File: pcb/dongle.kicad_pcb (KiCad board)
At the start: 2 copper layers, 12 x 16 mm, 28 parts, among them J1 USB_A, J2 Conn_01x01_Pin, J3 Conn_01x01_Pin, J4 Conn_01x01_Pin, J5 Conn_01x01_Pin, U3 nRF52833_QDxx, Y1 Crystal_GND24, Y2 Crystal_Small

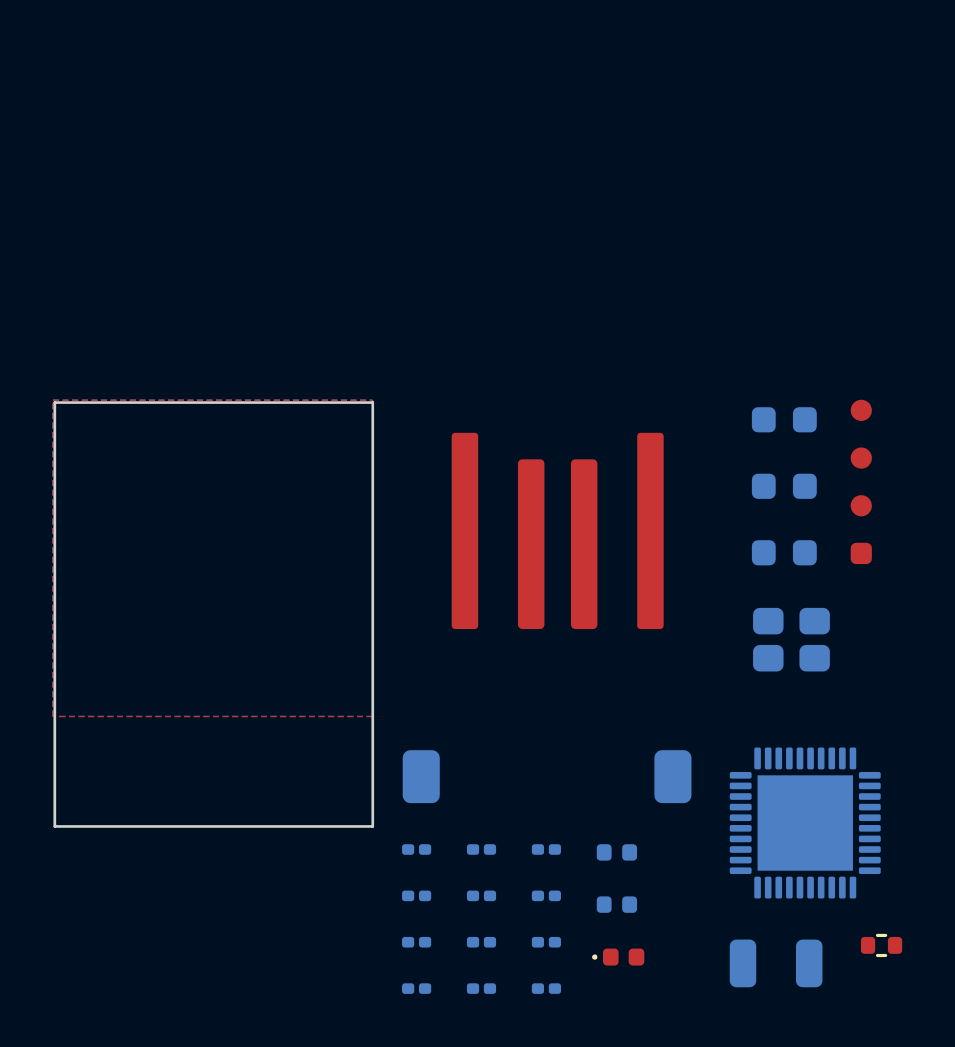
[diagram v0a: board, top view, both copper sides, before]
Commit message: update pcb
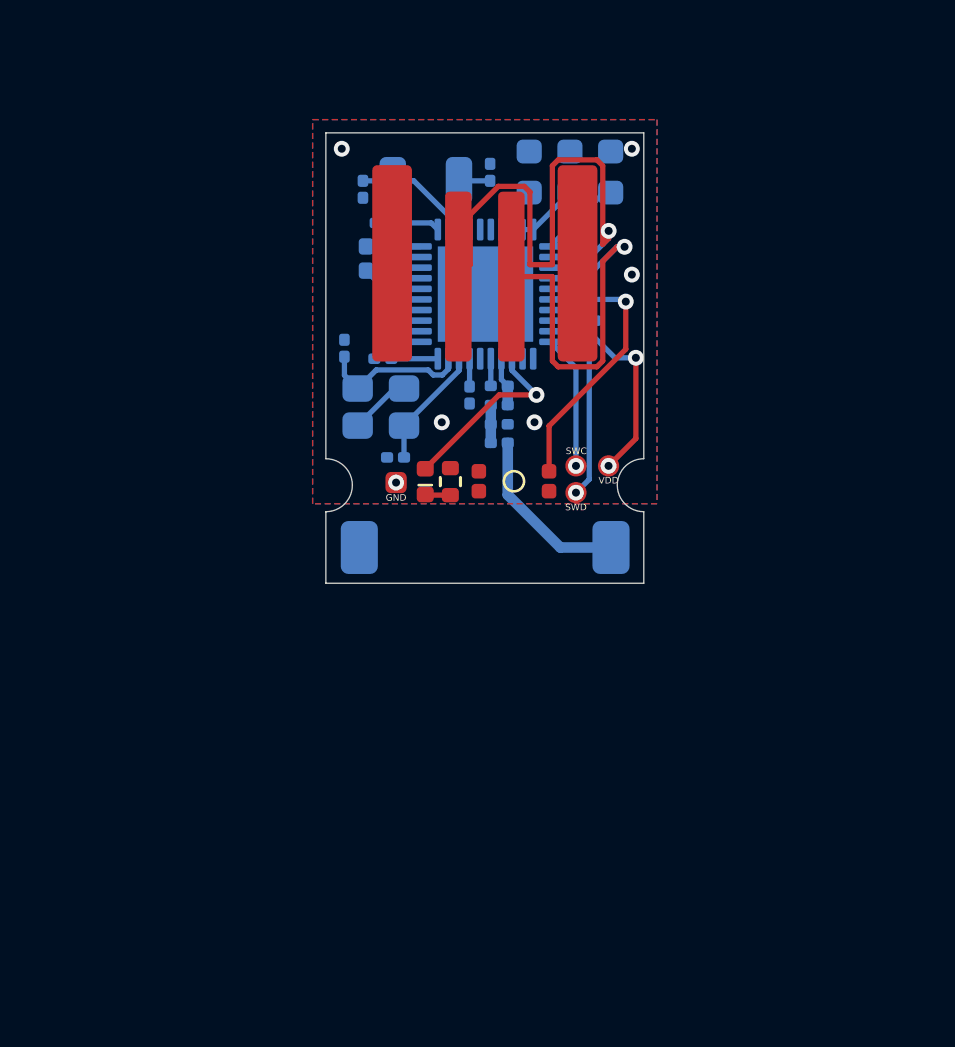
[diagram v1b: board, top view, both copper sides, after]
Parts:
- added SW1: SW_Push_45deg, dongle:SKTAAAE010, F.Cu at (157.1, 96.2)
- moved Y2 32.4 mm to (153.8, 84.8), turned to 180 degrees
- moved C16 27.6 mm to (151.4, 85.1), turned to -90 degrees
- moved C15 25.6 mm to (156.2, 84.5), turned to -90 degrees
- moved C13 25.6 mm to (152.0, 88.2), turned to 180 degrees
- moved C12 24.6 mm to (152.0, 87.3), turned to 180 degrees
- moved C11 24.1 mm to (152.2, 91.5), turned to 180 degrees
- moved C5 23.9 mm to (152.2, 86.4), turned to 180 degrees
- moved R1 23.9 mm to (154.7, 96.2), turned to 90 degrees
- moved U3 23.3 mm to (156.0, 89.1), turned to 90 degrees
- moved C7 22.1 mm to (159.8, 90.1)
- moved C4 21.5 mm to (156.5, 94.0), turned to 180 degrees
- moved C3 21.2 mm to (156.5, 92.5), turned to 180 degrees
- moved C2 20.8 mm to (150.7, 91.1), turned to 90 degrees
- moved L2 20.7 mm to (156.5, 94.7), turned to 180 degrees
- moved C10 20.7 mm to (155.4, 92.9), turned to -90 degrees
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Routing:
- net D-: track 0.00 -> 21.1 mm, vias 0 -> 1
- net D+: track 0.00 -> 14.8 mm, vias 0 -> 1
- net VDD: track 0.00 -> 12.9 mm, vias 0 -> 2
- net RESET: track 0.00 -> 10.5 mm, vias 0 -> 1
- net SWD: track 0.00 -> 7.15 mm, vias 0 -> 1
- net LED: track 0.00 -> 7.10 mm, vias 0 -> 1
- net Net-(AE1-A): track 0.00 -> 6.68 mm
- net XC2: track 0.00 -> 5.68 mm
- net SWC: track 0.00 -> 5.09 mm, vias 0 -> 1
- net GND: track 0.00 -> 4.70 mm, vias 0 -> 6
- net XC1: track 0.00 -> 4.58 mm
- net XL1: track 0.00 -> 4.30 mm
- net DECUSB: track 0.00 -> 3.13 mm
- net XL2: track 0.00 -> 3.01 mm
- net VBUS: track 0.00 -> 2.37 mm
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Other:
- board size 12 x 16 mm -> 12 x 17 mm

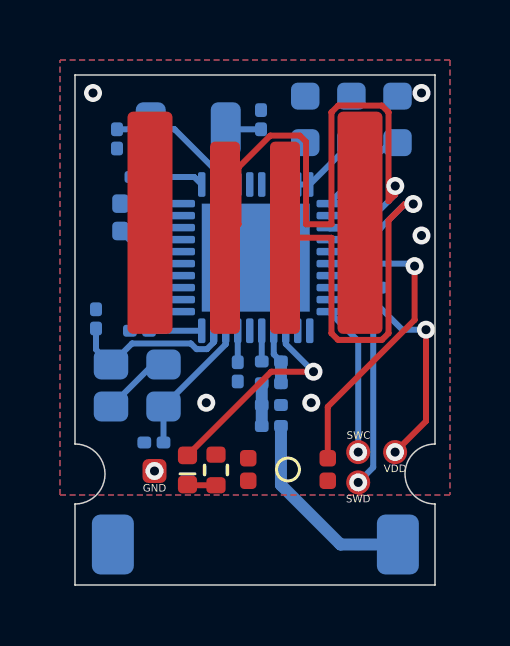
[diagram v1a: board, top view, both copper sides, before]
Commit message: some fix
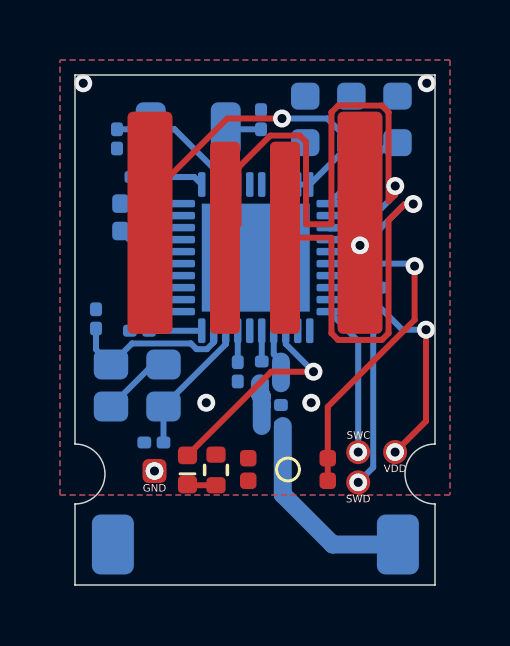
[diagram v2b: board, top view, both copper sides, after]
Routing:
- net VBUS: track 2.37 -> 11.4 mm, vias 0 -> 1
- net RESET: track 10.5 -> 11.2 mm
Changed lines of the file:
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@@
 			(outputformat 1)
 			(mirror no)
-			(drillshape 1)
+			(drillshape 0)
 			(scaleselection 1)
-			(outputdirectory "")
+			(outputdirectory "../../../../../dongle_gerber/")
 		)
 	)
@@
 	)
 	(footprint "dongle:QFN-40-1EP_5x5mm_P0.4mm_EP3.6x3.6mm"
-		(locked yes)
 		(layer "F.Cu")
 		(at 156.025 89.0875 90)
@@
 	)
 	(via micro
-		(at 150.6 83.6)
+		(at 159.5 88.68)
 		(size 0.6)
 		(drill 0.3)
 		(layers "F.Cu" "B.Cu")
-		(free yes)
 		(net 1)
 	)
 	(via micro
-		(at 157.875 93.925)
+		(at 150.275 83.275)
 		(size 0.6)
 		(drill 0.3)
@@
 	)
 	(via micro
-		(at 161.55 88.35)
+		(at 157.875 93.925)
 		(size 0.6)
 		(drill 0.3)
@@
 	)
 	(via micro
-		(at 161.55 83.6)
+		(at 161.724999 83.275)
 		(size 0.6)
 		(drill 0.3)
@@
 	)
 	(segment
+		(start 156.9 84.45)
+		(end 155.078756 84.45)
+		(width 0.2)
+		(layer "F.Cu")
+		(net 2)
+	)
+	(segment
+		(start 152.5 87.028756)
+		(end 152.5 87.925)
+		(width 0.2)
+		(layer "F.Cu")
+		(net 2)
+	)
+	(segment
+		(start 155.078756 84.45)
+		(end 152.5 87.028756)
+		(width 0.2)
+		(layer "F.Cu")
+		(net 2)
+	)
+	(via micro
+		(at 156.9 84.45)
+		(size 0.6)
+		(drill 0.3)
+		(layers "F.Cu" "B.Cu")
+		(net 2)
+	)
+	(segment
+		(start 159.2125 85.255)
+		(end 158.4075 84.45)
+		(width 0.2)
+		(layer "B.Cu")
+		(net 2)
+	)
+	(segment
+		(start 158.4075 84.45)
+		(end 156.9 84.45)
+		(width 0.2)
+		(layer "B.Cu")
+		(net 2)
+	)
+	(segment
 		(start 159.2125 85.255)
 		(end 159.2125 85.2625)
@@
 	)
 	(segment
-		(start 156.865 94.7)
-		(end 156.865 96.665)
-		(width 0.4)
+		(start 160.7625 98.65)
+		(end 158.59 98.65)
+		(width 0.6)
 		(layer "B.Cu")
 		(net 6)
 	)
 	(segment
-		(start 158.85 98.65)
-		(end 160.7625 98.65)
-		(width 0.4)
+		(start 158.59 98.65)
+		(end 156.926 96.986)
+		(width 0.6)
 		(layer "B.Cu")
 		(net 6)
 	)
 	(segment
-		(start 156.865 96.665)
-		(end 158.85 98.65)
-		(width 0.4)
+		(start 156.926 96.986)
+		(end 156.926 94.7)
+		(width 0.6)
 		(layer "B.Cu")
 		(net 6)
@@
 		(start 156.865 93.275)
 		(end 156.865 92.55)
-		(width 0.4)
+		(width 0.6)
 		(layer "B.Cu")
 		(net 9)
@@
 	)
 	(segment
-		(start 156.225 94)
-		(end 156.225 94.7)
-		(width 0.4)
+		(start 156.225 94.7)
+		(end 156.225 94)
+		(width 0.6)
 		(layer "B.Cu")
 		(net 11)
 	)
 	(segment
-		(start 156.225 93.275)
-		(end 156.225 94)
-		(width 0.4)
+		(start 156.225 93.698708)
+		(end 156.164 93.637708)
+		(width 0.6)
+		(layer "B.Cu")
+		(net 11)
+	)
+	(segment
+		(start 156.164 93.637708)
+		(end 156.164 93.275)
+		(width 0.6)
+		(layer "B.Cu")
+		(net 11)
+	)
+	(segment
+		(start 156.225 94)
+		(end 156.225 93.698708)
+		(width 0.6)
 		(layer "B.Cu")
 		(net 11)
@@
 		(width 0.2)
 		(layer "F.Cu")
+		(net 33)
+	)
+	(segment
+		(start 158.425 96.525)
+		(end 158.425 95.775)
+		(width 0.2)
+		(layer "F.Cu")

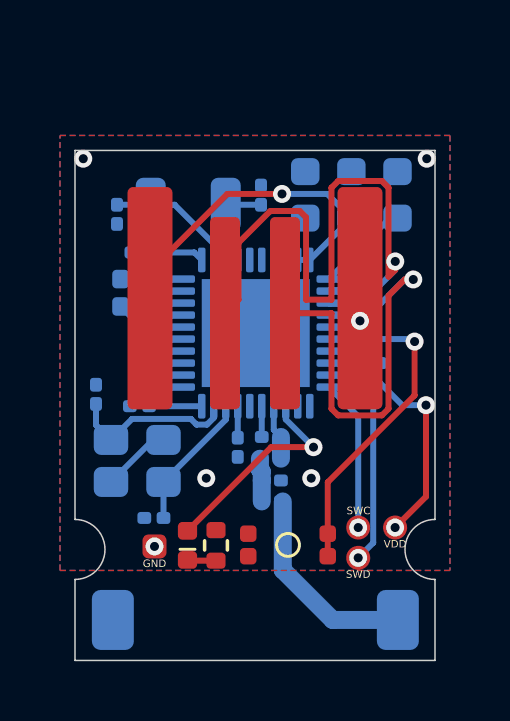
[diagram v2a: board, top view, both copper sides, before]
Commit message: fix routing
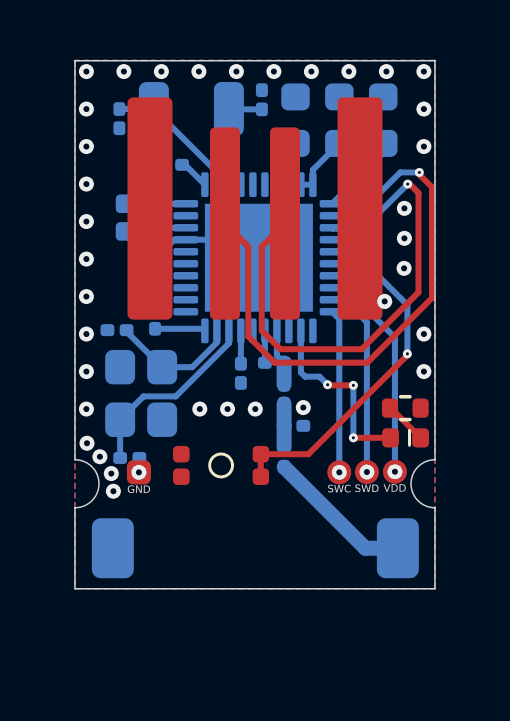
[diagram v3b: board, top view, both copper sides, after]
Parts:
- moved C11 8.77 mm to (160.1, 87.8), turned to -45 degrees
- moved D1 8.11 mm to (161.0, 92.6), turned to 180 degrees
- moved R1 7.79 mm to (161.0, 91.6), turned to 0 degrees
- moved C7 7.32 mm to (152.7, 88.6), turned to 90 degrees
- moved SW1 3.46 mm to (154.9, 93.5)
- moved Y2 3.19 mm to (153.9, 81.6)
- moved C16 3.19 mm to (151.5, 81.9)
- moved C15 3.18 mm to (156.2, 81.3)
- moved C5 3.10 mm to (153.2, 83.5)
- moved J1 2.99 mm to (154.8, 86.9)
- moved J4 2.87 mm to (159.7, 93.7)
- moved C19 2.53 mm to (160.3, 82.0)
- moved J5 2.52 mm to (152.1, 93.7)
- moved C17 2.52 mm to (158.8, 82.0)
- moved C12 2.51 mm to (152.1, 84.8)
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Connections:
- U3 pad 22: unconnected-(U3-NFC1/P0.09-Pad22) -> LED
- U3 pad 23: LED -> unconnected-(U3-NFC2/P0.10-Pad23)
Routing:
- net VBUS: track 11.4 -> 2.14 mm, vias 1 -> 0
- net D+: track 14.8 -> 17.1 mm
- net Net-(AE1-A): track 6.81 -> 4.92 mm
- net XC1: track 4.58 -> 6.37 mm
- net D-: track 21.1 -> 19.3 mm
- net XC2: track 5.68 -> 4.28 mm
- net LED: track 7.10 -> 6.30 mm, vias 1 -> 3
- net DEC1: track 1.81 -> 1.03 mm
- net SWD: track 7.15 -> 6.47 mm
- net XL2: track 3.01 -> 3.62 mm
- net RESET: track 11.2 -> 11.8 mm
- net GND: track 4.70 -> 5.10 mm, vias 6 -> 36
- net VDD: track 12.9 -> 12.8 mm, vias 2 -> 1
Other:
- board size 12 x 17 mm -> 12 x 17.6 mm
